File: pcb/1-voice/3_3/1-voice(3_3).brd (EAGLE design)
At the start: 72.6 x 30 mm, 128 parts, among them U1 STM32C8, U11 TL072, U12 TL072, U2 DAC084S085, U3 TLV760, U4 TL072, U5 TL072, U7 TL072, U9 TL072

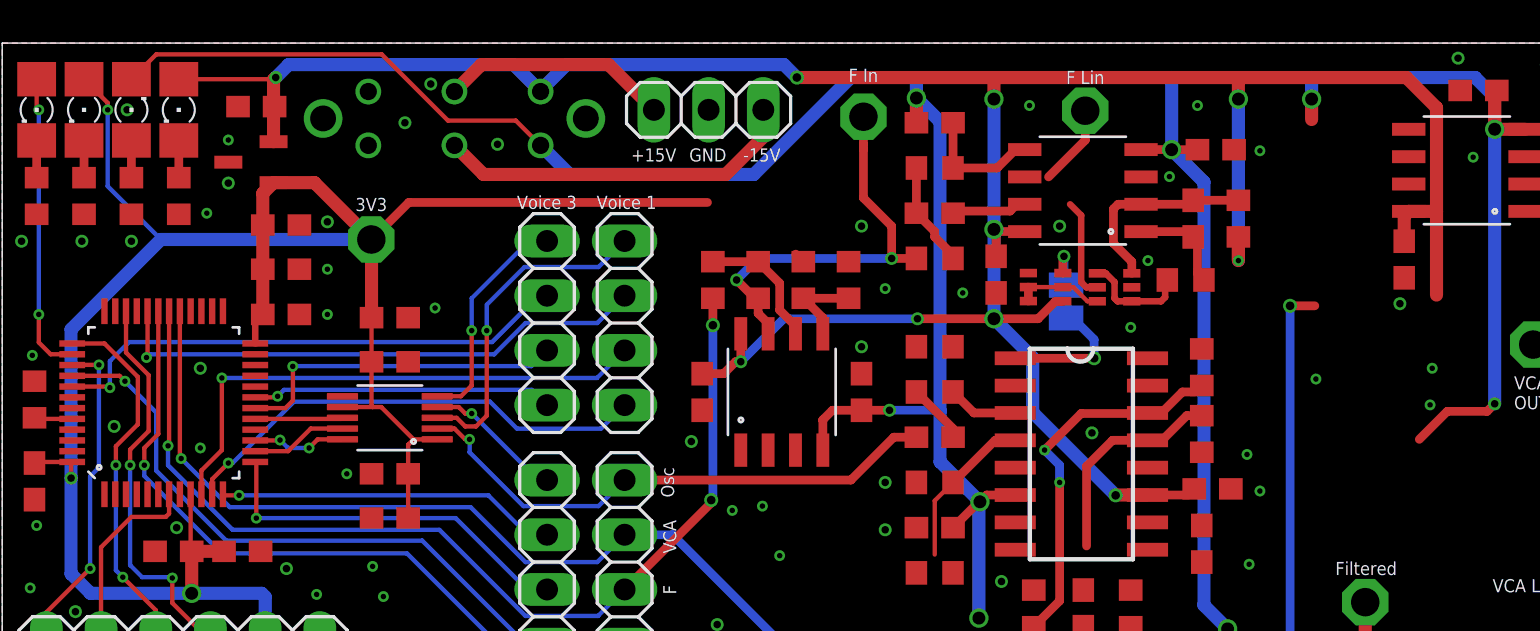
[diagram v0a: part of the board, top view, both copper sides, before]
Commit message: Standardize part vals
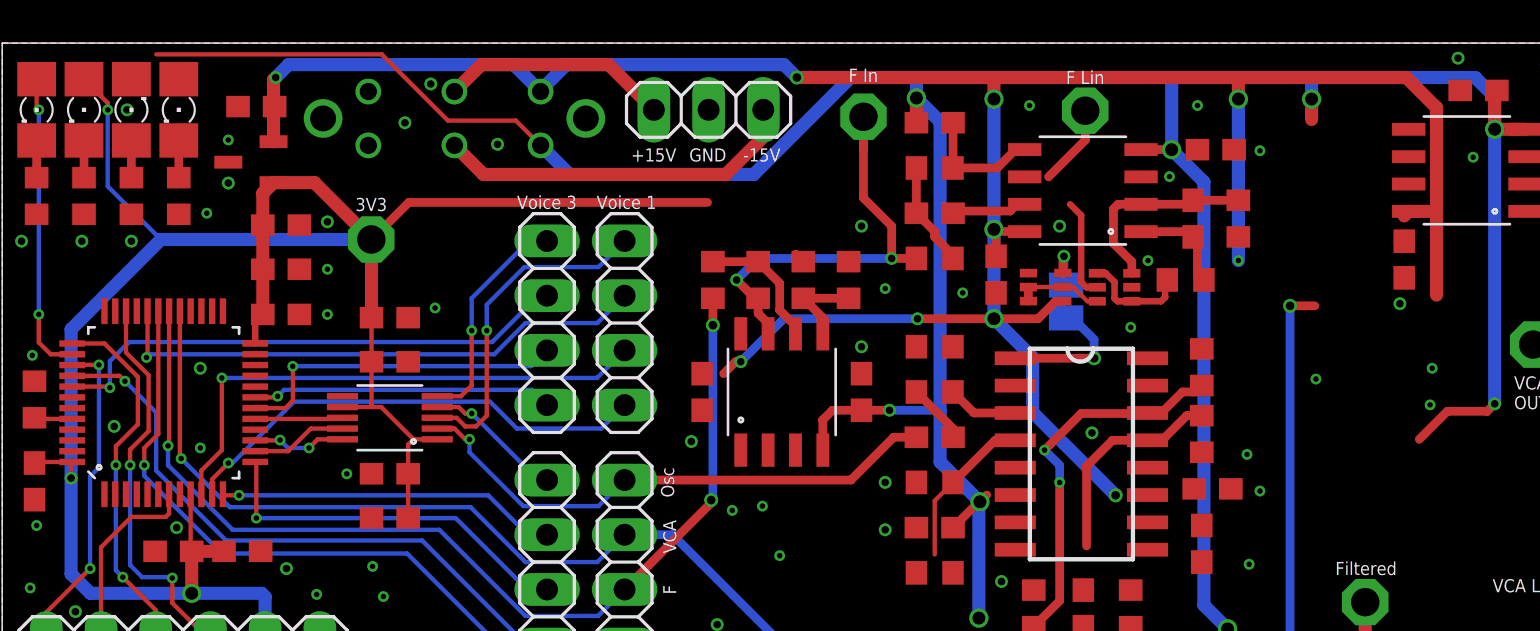
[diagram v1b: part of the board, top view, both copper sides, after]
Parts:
- removed TP8: TPPAD1-13, testpad:P1-13
- removed U$1: TRS, synth:TRS
- added JP2: (no value), pinhead:1X03
- added TP5: TPPAD1-13, testpad:P1-13
- C35, C36: value 2200p -> 2000p
- C9: value .01u -> 0.01u
- JP7: value (none) -> TRS; device pinhead:1X03 -> synth:TRS
- Q1, Q3: value (none) -> BC847BS
- Q2, Q4: value (none) -> BC857BS
- R1: value 3.5k -> 3.48k
- R15, R17: value 570 -> 562
- R41: value 1.6k -> 1.62k
- U6, U8: value (none) -> LM13700
- moved JP7 234.2 mm to (-31.8, -197.5), turned to 0 degrees
- moved TP6 26.3 mm to (52.7, 26.9)
- moved TP7 10.3 mm to (42.4, 26.6)
- renumbered C42 to C35, C43 to C36, C44 to C37, C45 to C38, JP10 to JP5, JP11 to JP6, JP8 to JP3, JP9 to JP4, U$6 to SW1, U12 to U10
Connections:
- net +15V renamed +12V
- net -15V renamed -12V
- new net N$3: R2.2, U8.14, VR2.1
- net -15V-IN: now also JP2.1; no longer JP7.1
- net 15V-IN: now also JP2.3; no longer JP7.3
- net F-CTRL0-LIN: now also TP6.TP; no longer TP7.TP
- net F0-OUT: now also TP5.TP; no longer R2.2, TP6.TP, U8.14, VR2.1
- net GND: now also JP2.2, JP7.P$1; no longer JP7.2, U$1.P$1
- net N$15: now also TP7.TP; no longer TP8.TP
- net VCA-OUT0: now also JP7.P$2; no longer U$1.P$2
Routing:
- net +12V: track 133.0 -> 120.5 mm
- net -12V: track 159.4 -> 155.2 mm
